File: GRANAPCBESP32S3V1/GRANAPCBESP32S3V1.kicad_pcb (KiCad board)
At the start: 2 copper layers, 3 parts, among them J1 Conn_01x14_Socket, P1 USB_C_Plug_USB2.0, U2 ESP32-S3-DevKitC

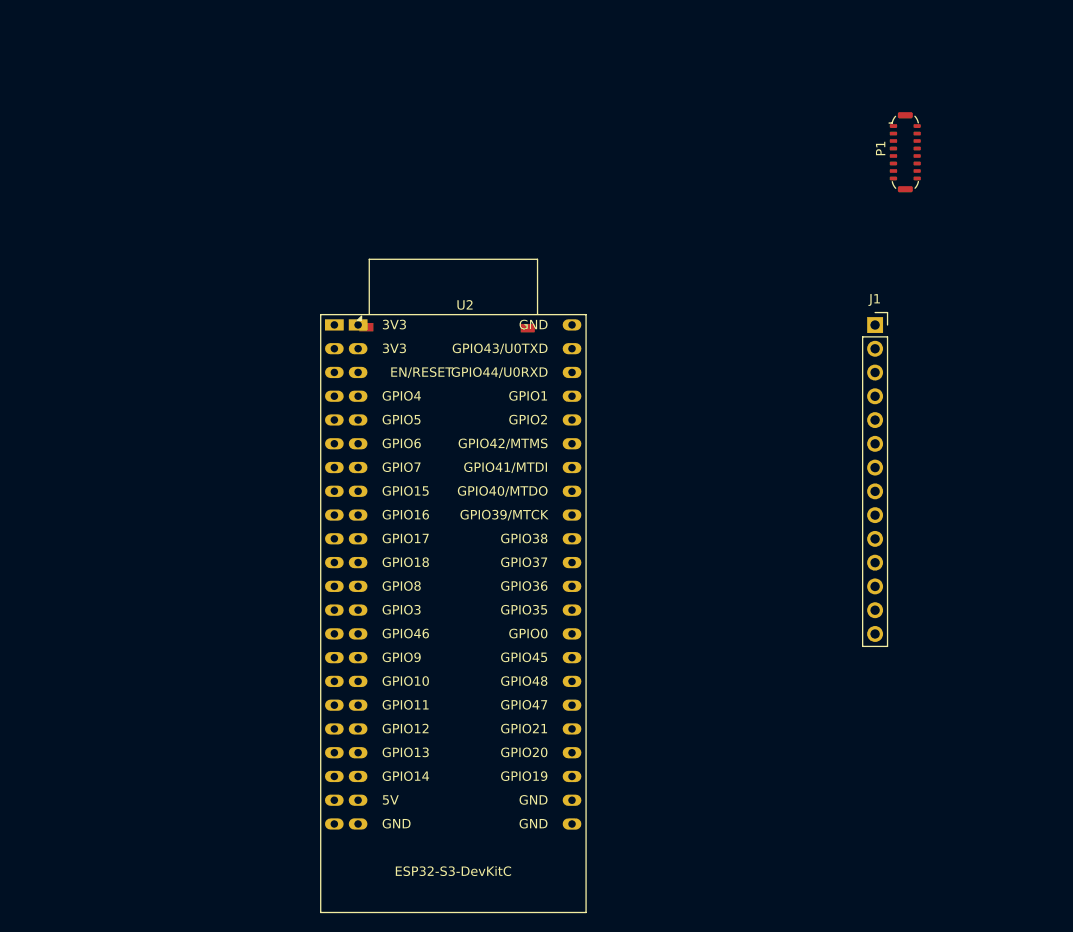
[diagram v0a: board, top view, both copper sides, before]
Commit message: Add files via upload
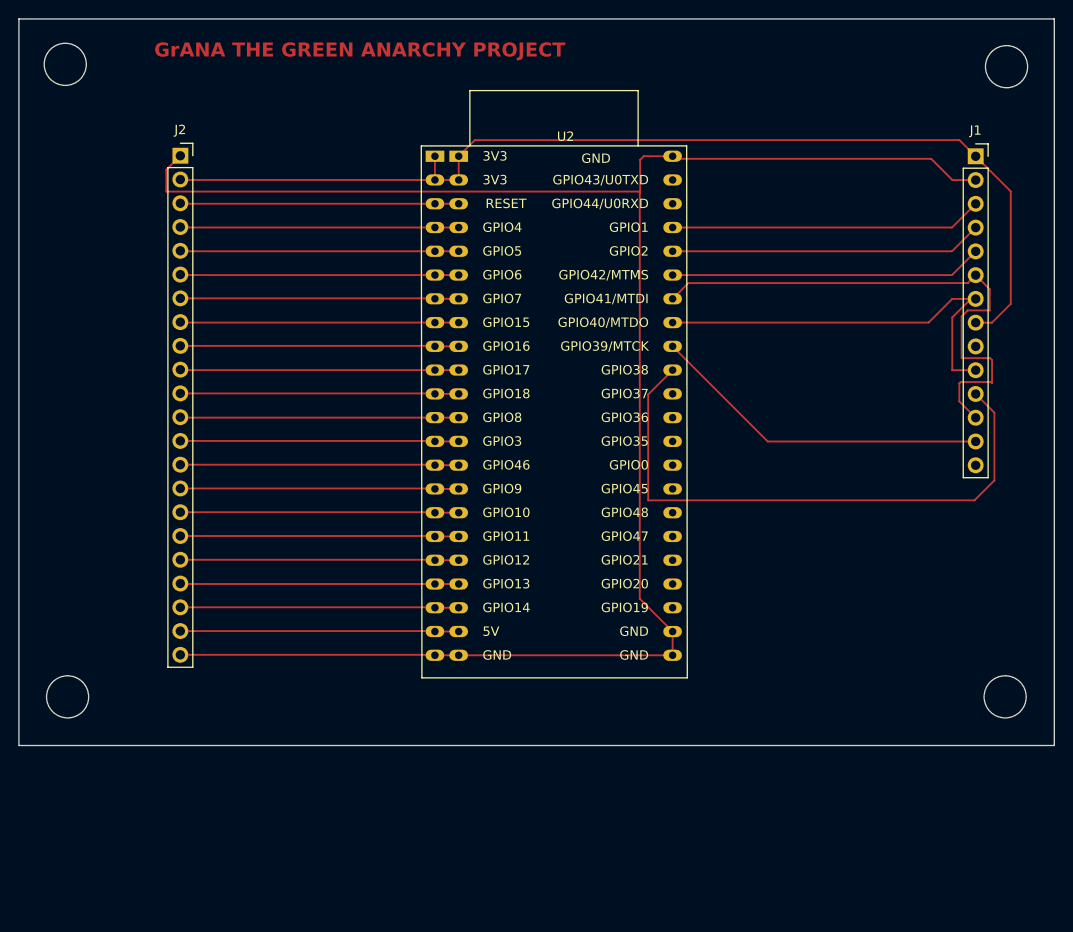
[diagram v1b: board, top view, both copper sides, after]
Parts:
- removed P1: USB_C_Plug_USB2.0, Connector_USB:USB_C_Plug_ShenzhenJingTuoJin_918-118A2021Y40002_Vertical
- added J2: Conn_01x22_Pin, Connector_PinSocket_2.54mm:PinSocket_1x22_P2.54mm_Vertical, F.Cu at (112.8, 57.7)
- added REF1: MountingHole_4.5mm, MountingHole:MountingHole_4.5mm, F.Cu at (100.5, 47.9)
- added REF2: MountingHole_4.5mm, MountingHole:MountingHole_4.5mm, F.Cu at (201.1, 48.1)
- added REF3: MountingHole_4.5mm, MountingHole:MountingHole_4.5mm, F.Cu at (100.7, 115.5)
- added REF4: MountingHole_4.5mm, MountingHole:MountingHole_4.5mm, F.Cu at (200.9, 115.5)
- moved J1 21.0 mm to (197.8, 57.7)
- moved U2 21.0 mm to (163.2, 69.0)
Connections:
- U2 pad 10: unconnected-(U2-GPIO17/ADC2_CH6-Pad10) -> Net-(J2-Pin_10)
- U2 pad 11: unconnected-(U2-GPIO18/ADC2_CH7-Pad11) -> Net-(J2-Pin_11)
- U2 pad 12: unconnected-(U2-GPIO8/ADC1_CH7-Pad12) -> Net-(J2-Pin_12)
- U2 pad 13: unconnected-(U2-GPIO3/ADC1_CH2-Pad13) -> Net-(J2-Pin_13)
- U2 pad 14: unconnected-(U2-GPIO46-Pad14) -> Net-(J2-Pin_14)
- U2 pad 15: unconnected-(U2-GPIO9/ADC1_CH8-Pad15) -> Net-(J2-Pin_15)
- U2 pad 16: unconnected-(U2-GPIO10/ADC1_CH9-Pad16) -> Net-(J2-Pin_16)
- U2 pad 17: unconnected-(U2-GPIO11/ADC2_CH0-Pad17) -> Net-(J2-Pin_17)
- U2 pad 18: unconnected-(U2-GPIO12/ADC2_CH1-Pad18) -> Net-(J2-Pin_18)
- U2 pad 19: unconnected-(U2-GPIO13/ADC2_CH2-Pad19) -> Net-(J2-Pin_19)
- U2 pad 20: unconnected-(U2-GPIO14/ADC2_CH3-Pad20) -> Net-(J2-Pin_20)
- U2 pad 26: Net-(P1-D-) -> Net-(P1-CC)
- U2 pad 3: unconnected-(U2-CHIP_PU-Pad3) -> Net-(J2-Pin_3)
- U2 pad 4: unconnected-(U2-GPIO4/ADC1_CH3-Pad4) -> Net-(J2-Pin_4)
- U2 pad 5: unconnected-(U2-GPIO5/ADC1_CH4-Pad5) -> Net-(J2-Pin_5)
- U2 pad 6: unconnected-(U2-GPIO6/ADC1_CH5-Pad6) -> Net-(J2-Pin_6)
- U2 pad 7: unconnected-(U2-GPIO7/ADC1_CH6-Pad7) -> Net-(J2-Pin_7)
- U2 pad 8: Net-(P1-D-) -> Net-(J2-Pin_8)
- U2 pad 9: Net-(P1-D+) -> Net-(J2-Pin_9)
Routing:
- net Net-(J1-Pin_2): track 0.00 -> 199.3 mm
- net Net-(J1-Pin_1): track 0.00 -> 114.4 mm
- net Net-(J1-Pin_11): track 0.00 -> 63.0 mm
- net Net-(J1-Pin_12): track 0.00 -> 59.3 mm
- net Net-(J1-Pin_10): track 0.00 -> 44.9 mm
- net Net-(J1-Pin_13): track 0.00 -> 36.6 mm
- net Net-(J1-Pin_5): track 0.00 -> 33.4 mm
- net Net-(J1-Pin_4): track 0.00 -> 33.4 mm
- net Net-(J1-Pin_3): track 0.00 -> 33.4 mm
- net Net-(J2-Pin_9): track 0.00 -> 29.8 mm
- net Net-(J2-Pin_18): track 0.00 -> 29.8 mm
- net Net-(J2-Pin_11): track 0.00 -> 29.8 mm
- net Net-(J2-Pin_8): track 0.00 -> 29.8 mm
- net Net-(J2-Pin_6): track 0.00 -> 29.8 mm
- net Net-(J2-Pin_5): track 0.00 -> 29.8 mm
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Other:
- board outline added: 110.7 x 77.7 mm
- board text added: "GrANA THE GREEN ANARCHY PROJECT"
